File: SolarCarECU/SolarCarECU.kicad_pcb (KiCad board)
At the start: 2 copper layers, 160 x 100.3 mm, 104 parts, among them J1 Screw_Terminal_01x02, J2 USB_B_Micro, J3 Screw_Terminal_01x04, J4 Screw_Terminal_01x08, J5 Screw_Terminal_01x08, J6 Screw_Terminal_01x14, J7 Screw_Terminal_01x14, Q1 QM6015D, Q2 PZT2222A, Q3 QM6015D, Q4 QM6015D, Q5 QM6015D, Q6 QM6015D, U1 Teensy3.6, U10 LM324A, U2 EL7202CN, U3 EL7202CN, U4 L7805, U5 MCP2562-E-P, U6 MCP2562-E-P, U7 4504, U8 4504, U9 4504

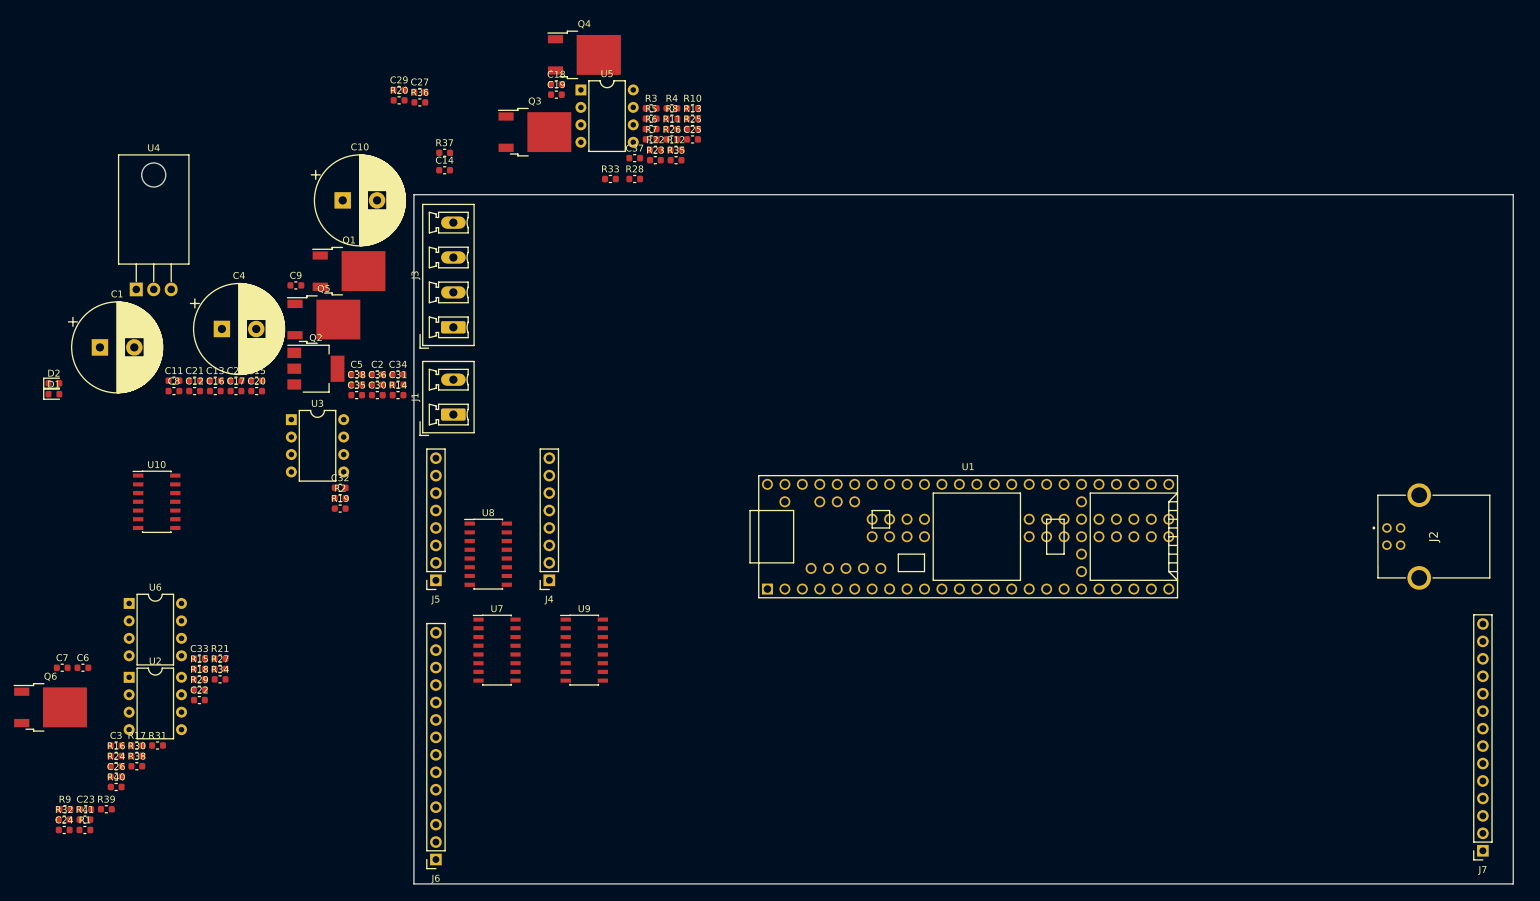
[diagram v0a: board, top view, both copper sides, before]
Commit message: begun layout of PCB
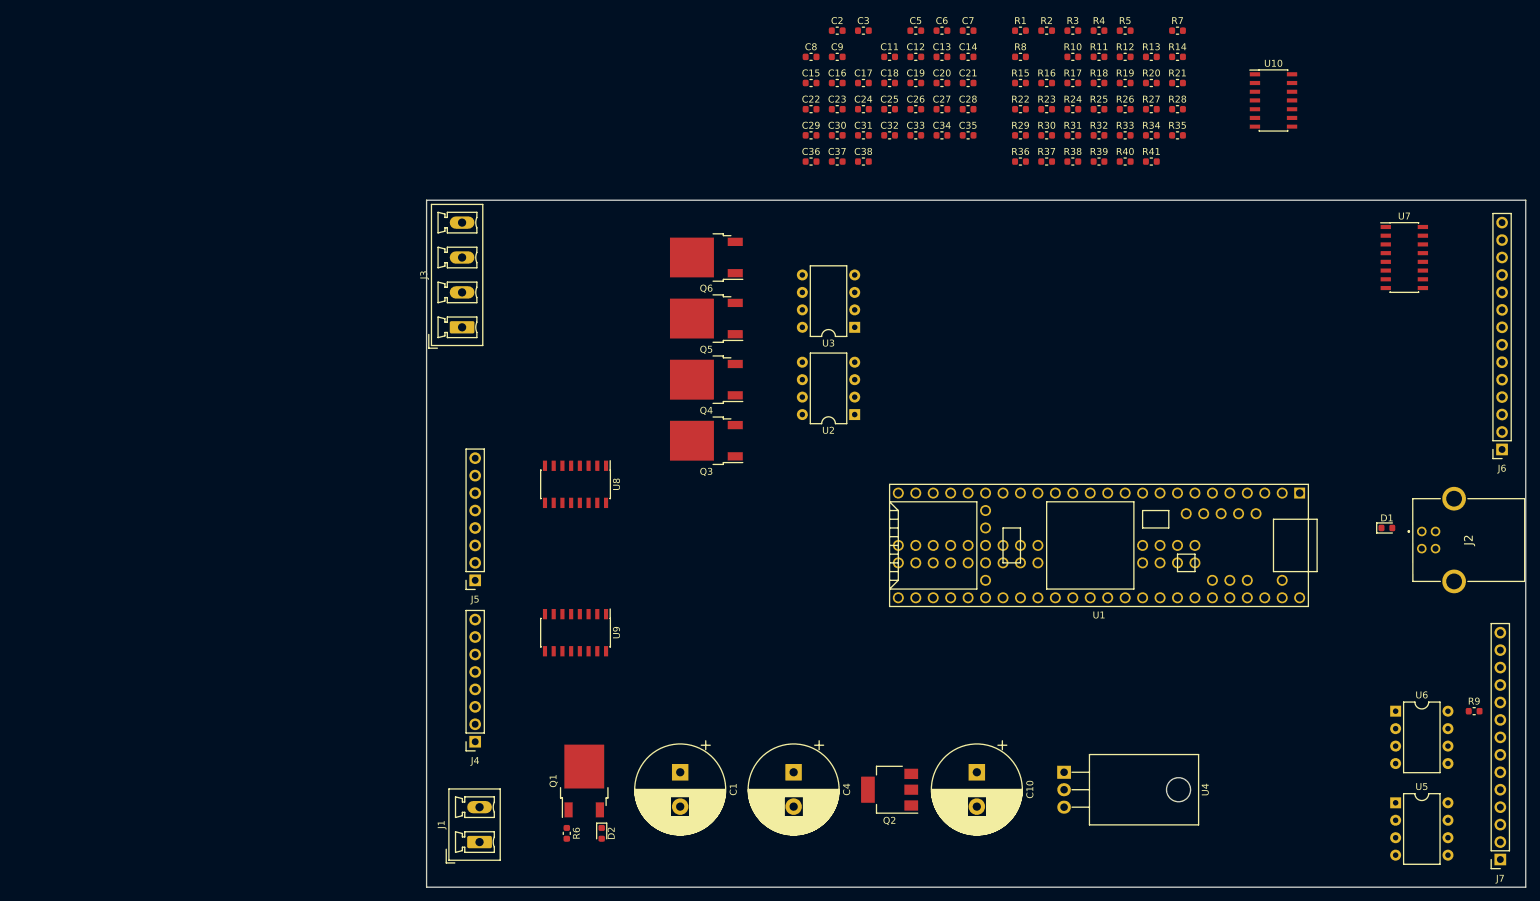
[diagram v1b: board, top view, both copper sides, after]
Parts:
- moved R9 205.6 mm to (237.5, 119.4)
- moved D1 195.0 mm to (224.8, 92.7)
- moved U6 185.0 mm to (226.1, 119.4)
- moved R41 182.4 mm to (190.5, 39.4)
- moved R32 180.6 mm to (182.9, 35.6)
- moved R1 179.1 mm to (171.4, 20.3)
- moved R40 172.8 mm to (186.7, 39.4)
- moved U10 172.7 mm to (208.3, 30.5)
- moved R39 172.5 mm to (182.9, 39.4)
- moved R24 168.9 mm to (179.1, 31.8)
- moved R16 167.1 mm to (175.3, 27.9)
- moved R17 166.9 mm to (179.1, 27.9)
- moved J6 166.3 mm to (241.6, 81.3)
- moved R21 162.6 mm to (194.3, 27.9)
- moved R38 162.2 mm to (179.1, 39.4)
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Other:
- board size 160 x 100.3 mm -> 160 x 100 mm
